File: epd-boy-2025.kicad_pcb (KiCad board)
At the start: 2 copper layers, 32.5 x 64.5 mm, 43 parts, among them J1 FH12A-24S-0.5SH(55), Q1 SI1308EDL-T1-GE3, SW1 SW_Push, SW10 SW_SPDT, SW2 SW_Push, SW3 SW_Push, SW4 SW_Push, SW5 SW_Push, SW6 SW_Push, SW7 SW_Push, SW8 SW_Push, SW9 SW_Push, U1 xiao-ble, U2 DW01A, U3 FS8205

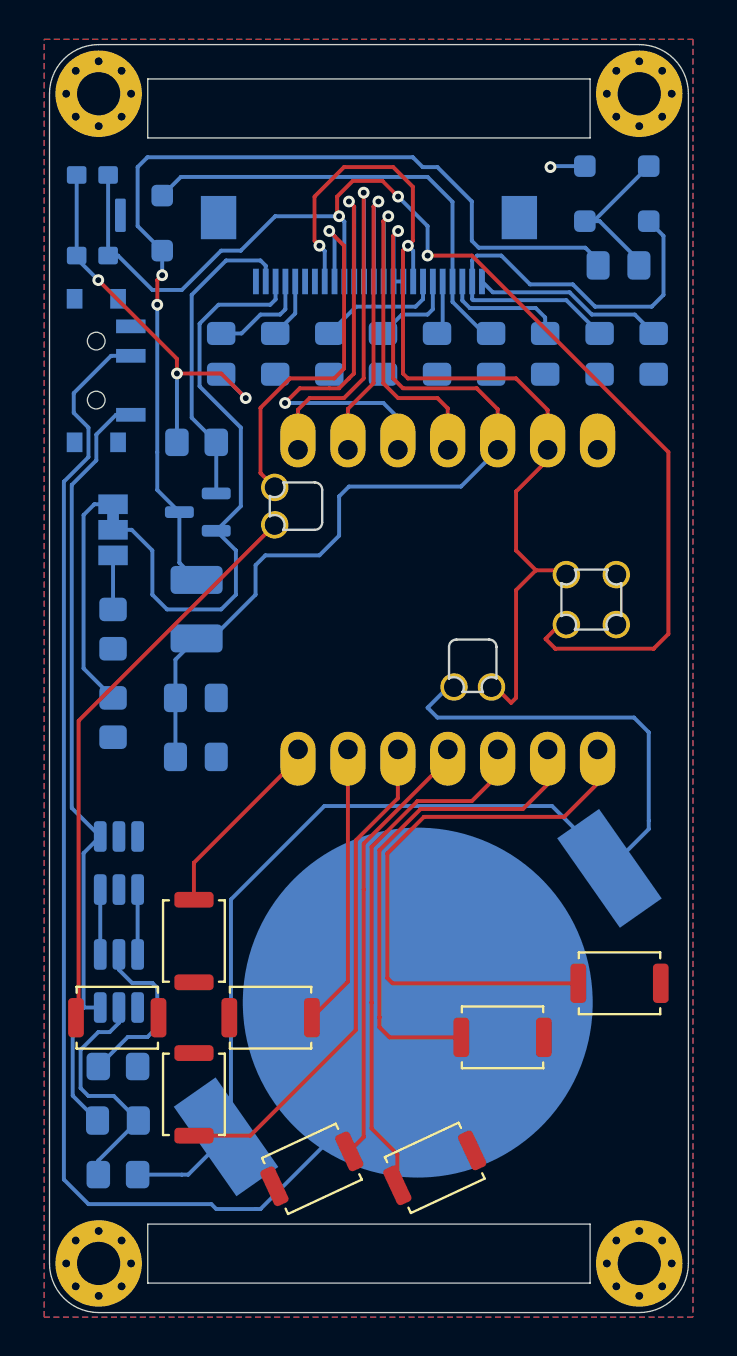
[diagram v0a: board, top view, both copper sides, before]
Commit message: Revision
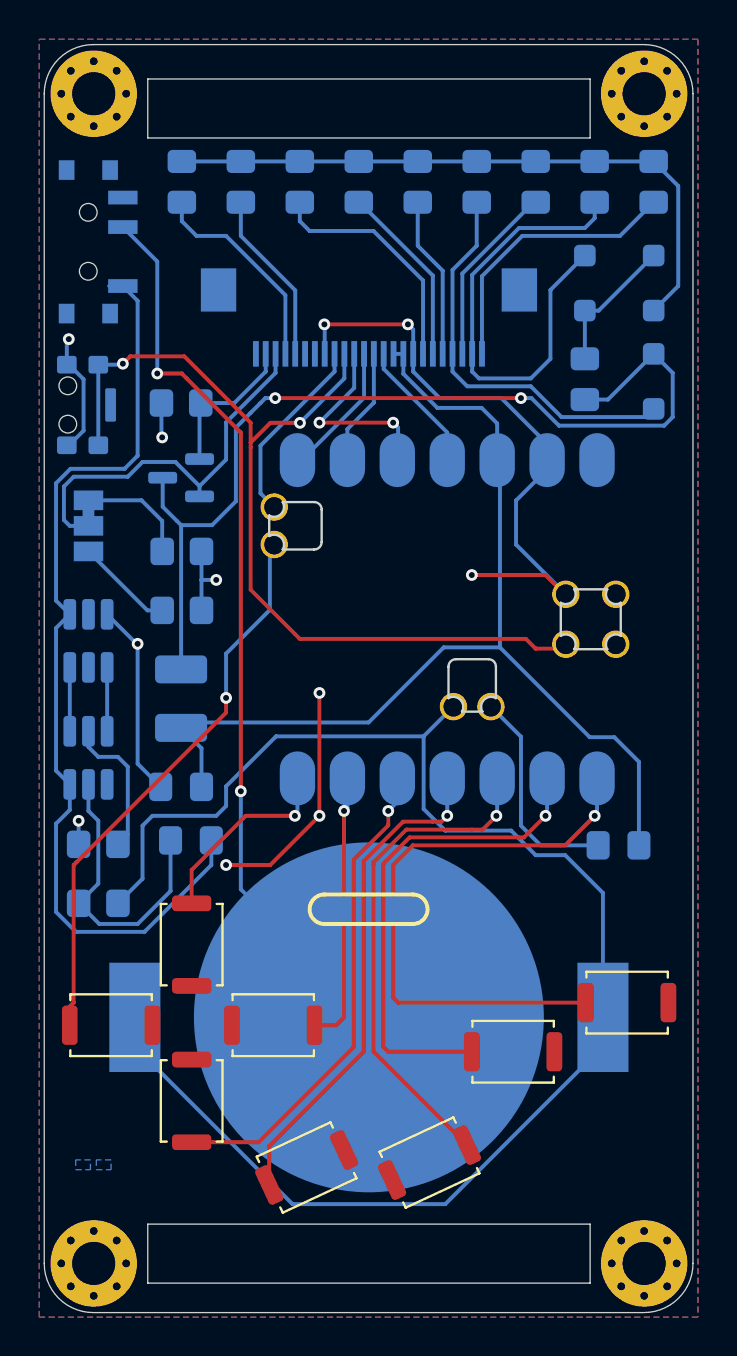
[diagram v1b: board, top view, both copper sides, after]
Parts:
- removed the REF** at (130.0, 27.5)
- removed the REF** at (130.0, 87.0)
- removed the REF** at (102.5, 87.0)
- removed the REF** at (102.5, 27.5)
- added REF**: MountingHole_2.2mm_M2_Pad_Via, MountingHole:MountingHole_2.2mm_M2_Pad_Via, F.Cu at (130.3, 87.0)
- added REF**: MountingHole_2.2mm_M2_Pad_Via, MountingHole:MountingHole_2.2mm_M2_Pad_Via, F.Cu at (102.3, 87.0)
- added REF**: MountingHole_2.2mm_M2_Pad_Via, MountingHole:MountingHole_2.2mm_M2_Pad_Via, F.Cu at (130.3, 27.5)
- added REF**: MountingHole_2.2mm_M2_Pad_Via, MountingHole:MountingHole_2.2mm_M2_Pad_Via, F.Cu at (102.3, 27.5)
- SW9: footprint Button_Switch_SMD:SW_SPST_CK_KMS2xxG -> Button_Switch_SMD:SW_SPST_CK_KMS2xxGP
- moved D2 26.3 mm to (130.8, 42.1), turned to 90 degrees
- moved C11 22.0 mm to (129.0, 65.8), turned to 0 degrees
- moved C13 14.7 mm to (107.2, 65.5), turned to 0 degrees
- moved R4 13.8 mm to (102.5, 68.7)
- moved U2 11.5 mm to (102.0, 61.3)
- moved U3 11.4 mm to (102.0, 55.4)
- moved R5 11.3 mm to (102.5, 65.7), turned to 180 degrees
- moved SW9 9.66 mm to (101.7, 43.4)
- moved R2 9.15 mm to (106.8, 50.8), turned to 180 degrees
- moved C10 8.98 mm to (106.8, 32.0), turned to -90 degrees
- moved C9 8.92 mm to (109.8, 32.0), turned to -90 degrees
- moved C1 8.88 mm to (112.8, 32.0), turned to -90 degrees
- moved C2 8.84 mm to (115.8, 32.0), turned to -90 degrees
- moved C3 8.80 mm to (118.8, 32.0), turned to -90 degrees
- moved C4 8.78 mm to (121.8, 32.0), turned to -90 degrees
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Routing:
- net GND: track 72.4 -> 109.1 mm, vias 6 -> 11
- net Net-(BT1--): track 69.0 -> 46.1 mm, vias 0 -> 2
- net EP_RST: track 63.5 -> 46.3 mm, vias 3 -> 2
- net BAT+: track 61.2 -> 77.4 mm
- net EP_DC: track 24.8 -> 10.5 mm
- net EP_CS: track 20.0 -> 7.28 mm, vias 1 -> 0
- net EP_CLK: track 17.4 -> 6.44 mm, vias 1 -> 0
- net EP_MOSI: track 17.9 -> 7.22 mm, vias 1 -> 0
- net Net-(J1-Pin_3): track 30.4 -> 19.9 mm
- net EP_BUSY: track 19.1 -> 9.34 mm, vias 1 -> 0
- net Net-(SW10-A): track 40.1 -> 48.6 mm
- net Net-(J1-Pin_2): track 16.0 -> 7.75 mm
- net +3V3: track 46.6 -> 53.9 mm, vias 1 -> 0
- net Net-(JP1-A): track 11.6 -> 5.73 mm
- net Net-(J1-Pin_18): track 6.39 -> 12.2 mm
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- added copper zone on B.Cu, net (none)
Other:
- board size 32.5 x 64.5 mm -> 33 x 64.5 mm
- board text added: "0.47R"
- board text added: "100R"
- board text added: "100nF"
- board text added: "10K"
- board text added: "1K"
- board text added: "3R"
- board text added: "4.7uF"
- board text added: "DW01A"
- board text added: "FS8205"
